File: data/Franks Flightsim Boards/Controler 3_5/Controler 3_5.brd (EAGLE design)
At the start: 80 x 65 mm, 24 parts, among them IC1 SN65HVD230, IC2 LOLIN32LITE, IC3 LD117AV33, IC4 7805T, J1 External, J2 FEMALE 2x3, X1 BUS

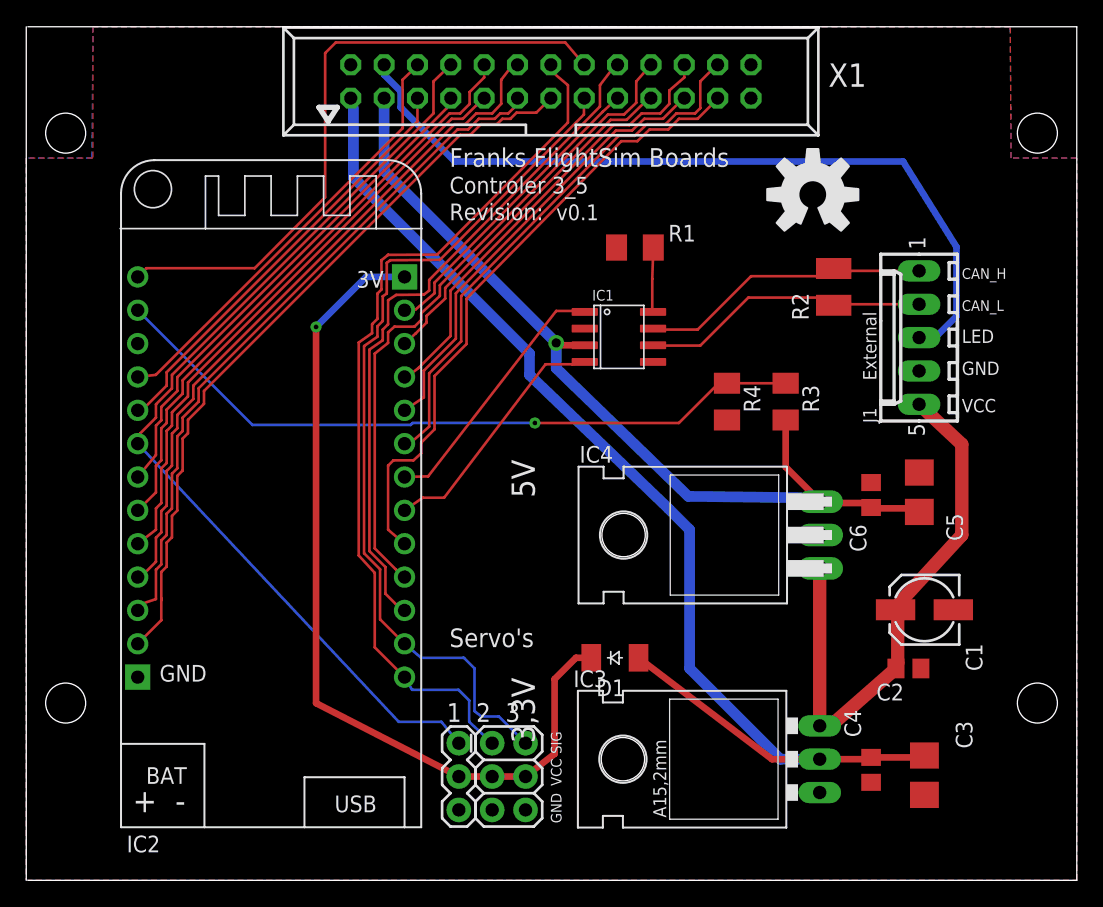
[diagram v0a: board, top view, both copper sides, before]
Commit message: Update dev status
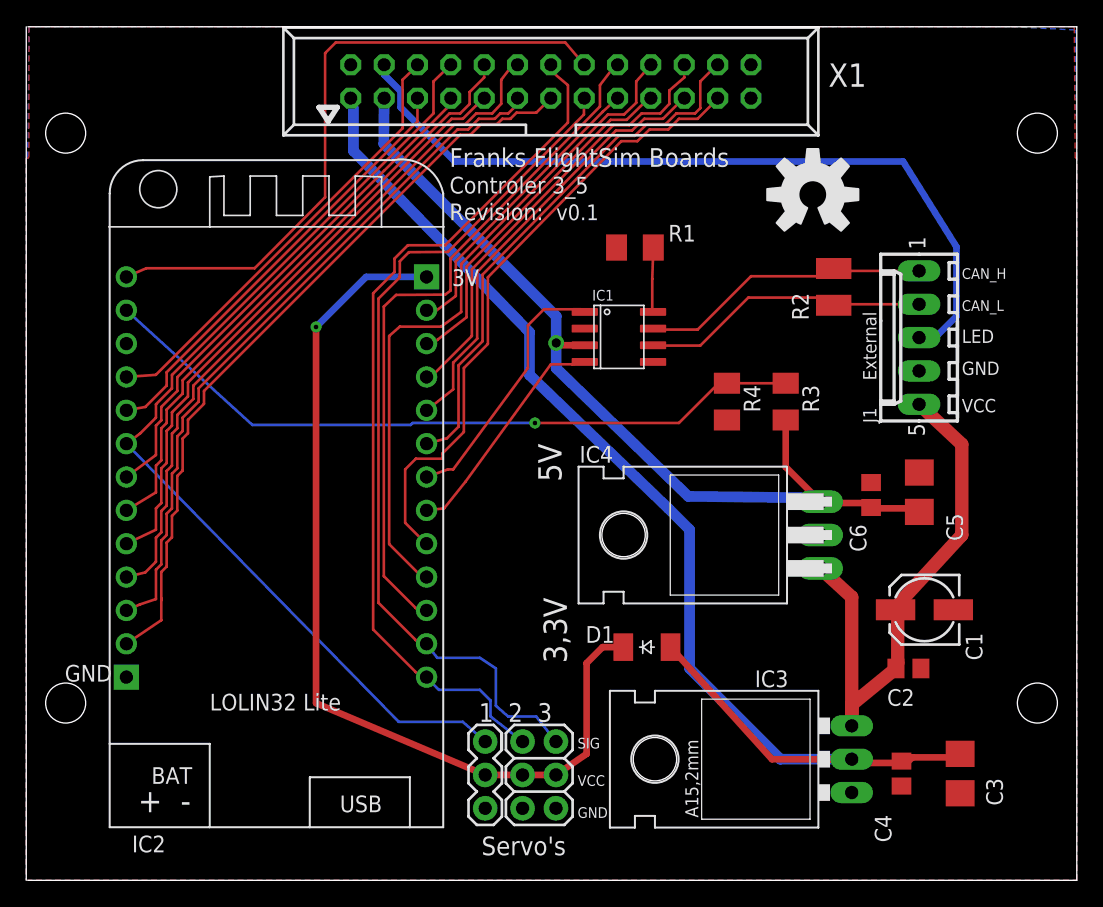
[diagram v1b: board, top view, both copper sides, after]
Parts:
- moved J3 5.58 mm to (35.0, 10.6), turned to 270 degrees
- moved C3 2.72 mm to (71.1, 8.13)
- moved D1 2.57 mm to (47.3, 17.8)
- moved IC3 2.44 mm to (59.1, 9.22)
- moved C4 2.33 mm to (66.6, 8.13)
- moved J2 2.32 mm to (37.8, 10.6)
- moved IC2 0.41 mm to (19.1, 25.6)
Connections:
- net GND: now also J3.3; no longer J3.1
- net P32: now also J3.1; no longer J3.3
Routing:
- net 3_3V: track 91.5 -> 97.9 mm
- net 3_3V_DIODE: track 66.2 -> 71.1 mm
- net P32: track 73.1 -> 76.0 mm
- net CAN_R: track 19.1 -> 17.6 mm
- net P00: track 50.3 -> 51.3 mm
- net P34: track 33.3 -> 34.1 mm
- net P35: track 32.7 -> 33.6 mm
- net P02: track 51.9 -> 52.8 mm
- net P27: track 52.3 -> 53.1 mm
- net P26: track 45.5 -> 46.2 mm
- net P36: track 48.6 -> 49.4 mm
- net P18: track 34.3 -> 33.6 mm
- net P25: track 45.3 -> 46.0 mm
- net P12: track 57.0 -> 57.7 mm
- net P14: track 52.8 -> 53.5 mm
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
